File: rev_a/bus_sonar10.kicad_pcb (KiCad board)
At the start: 2 copper layers, 100 x 50 mm, 63 parts, among them J1 POWER_SELECT, J2 TERMINATE_JUMPER, SW1 MJTP1243, U1 LM2940, U2 LTV-826, U3 LTV-826, U4 LTV-826, U5 754410, U6 LM2940, U7 74HCT08, U8 MCP2562, U9 ATMEGA328_DIP28, X1 CRYSTAL

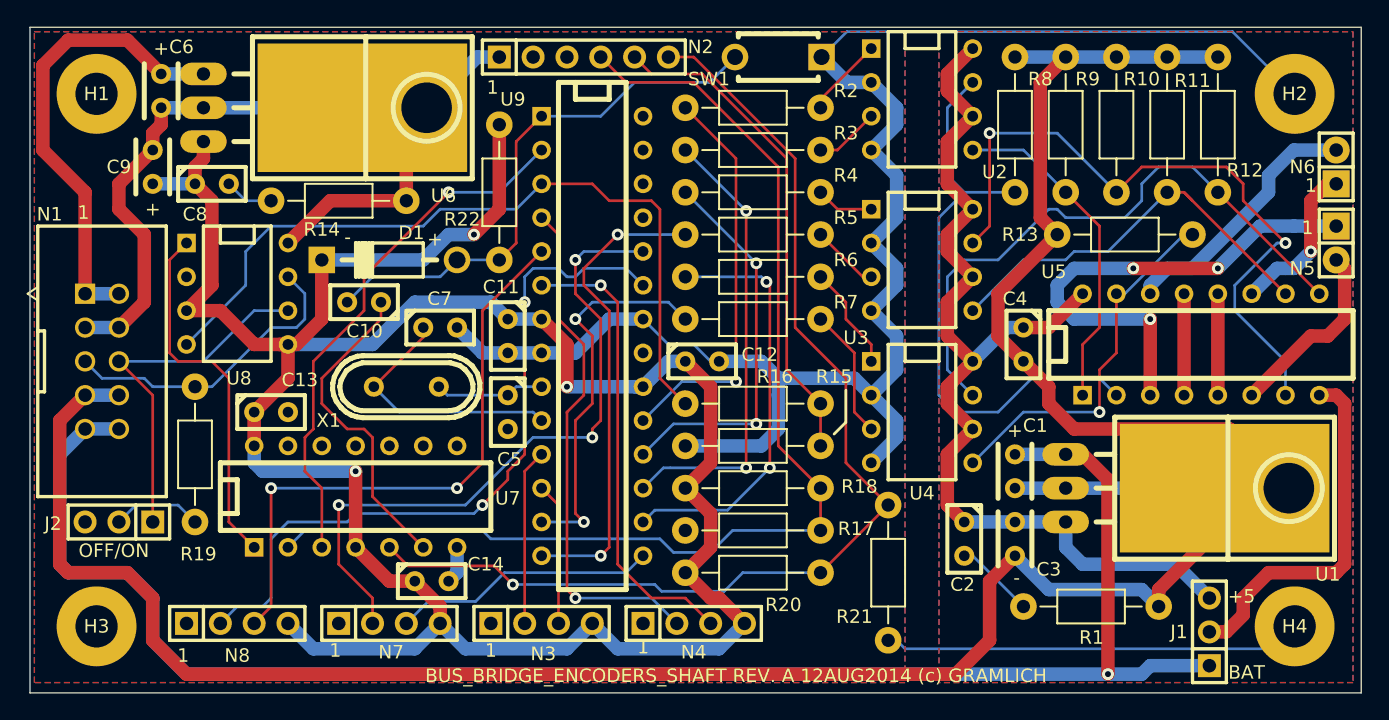
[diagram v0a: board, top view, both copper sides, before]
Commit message: Finnished laying out Rev. A
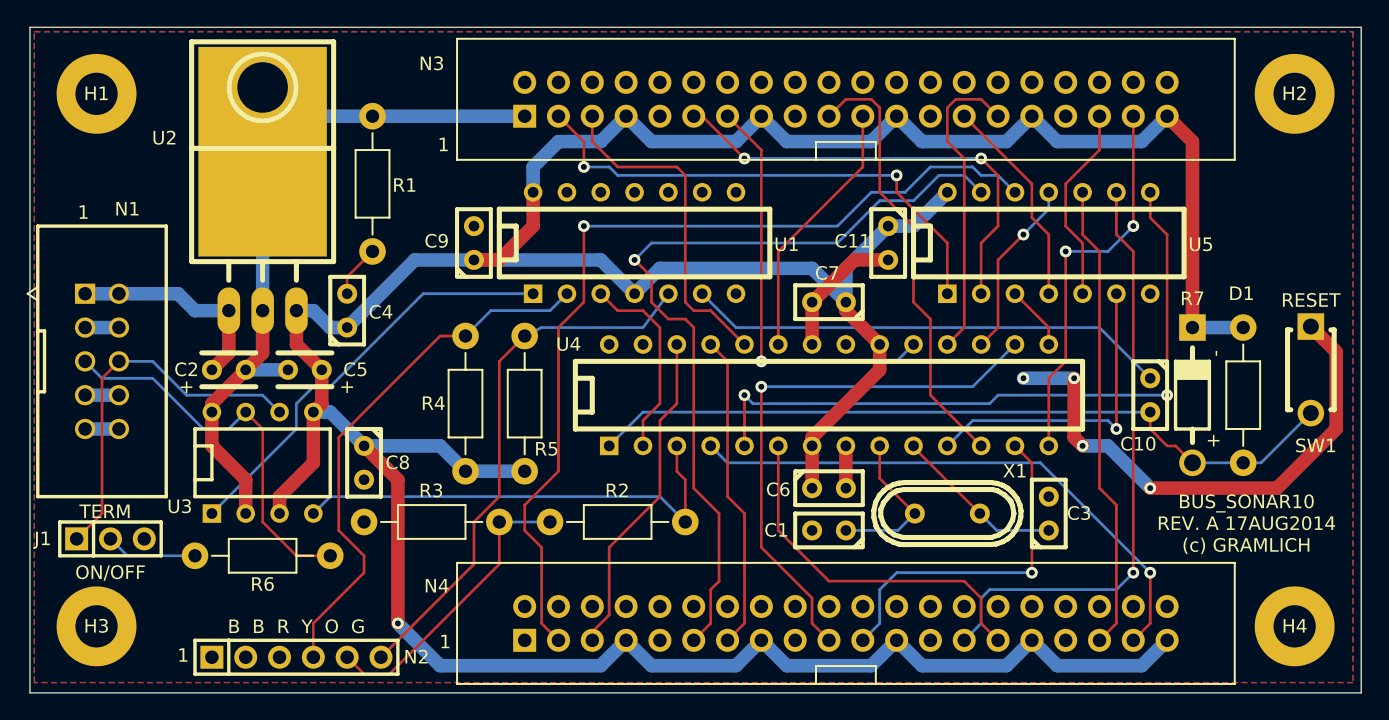
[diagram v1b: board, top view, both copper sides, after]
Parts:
- removed C12, C13, C14: .1uF, Bus_Bridge_Encoders_Sonar_Rev_A:Capacitor3MMDiscRM2.5
- removed J2: TERMINATE_JUMPER, Bus_Bridge_Encoders_Sonar_Rev_A:Pin_Header_Straight_1x03
- removed N5, N6: MOTOR_CONNECTOR, Bus_Bridge_Encoders_Sonar_Rev_A:Pin_Header_Straight_1x02
- removed N7, N8: HC_SR04_CONNECTOR, Bus_Bridge_Encoders_Sonar_Rev_A:Pin_Header_Straight_1x04
- removed R10, R11, R12, R13, R22, R8, R9: 10K, Bus_Bridge_Encoders_Sonar_Rev_A:Resistor_Horizontal_400
- removed R14, R19: .47, Bus_Bridge_Encoders_Sonar_Rev_A:Resistor_Horizontal_400
- removed R15, R17, R20: 22K, Bus_Bridge_Encoders_Sonar_Rev_A:Resistor_Horizontal_400
- removed R16, R18, R21: 33K, Bus_Bridge_Encoders_Sonar_Rev_A:Resistor_Horizontal_400
- removed U6: LM2940, Bus_Bridge_Encoders_Sonar_Rev_A:TO-220_Neutral123_Horizontal_LargePads
- removed U7: 74HCT08, Bus_Bridge_Encoders_Sonar_Rev_A:DIP-14__300
- removed U8: MCP2562, Bus_Bridge_Encoders_Sonar_Rev_A:DIP-8__300
- removed U9: ATMEGA328_DIP28, Bus_Bridge_Encoders_Sonar_Rev_A:DIP-28__300
- C1, C3: value 22uF -> 18pF; footprint Bus_Bridge_Encoders_Sonar_Rev_A:Capacitor4x3RM2-5_RevB -> Bus_Sonar10_Rev_A:Capacitor3MMDiscRM2.5
- C10: value .1uF -> 1uF; footprint Bus_Bridge_Encoders_Sonar_Rev_A:Capacitor3MMDiscRM2.5 -> Bus_Sonar10_Rev_A:Capacitor3MMDiscRM2.5
- C11, C4, C8: footprint Bus_Bridge_Encoders_Sonar_Rev_A:Capacitor3MMDiscRM2.5 -> Bus_Sonar10_Rev_A:Capacitor3MMDiscRM2.5
- C2: value .1uF -> 22uF; footprint Bus_Bridge_Encoders_Sonar_Rev_A:Capacitor3MMDiscRM2.5 -> Bus_Sonar10_Rev_A:Capacitor4x3RM2-5_RevB
- C5: value 18pF -> 22uF; footprint Bus_Bridge_Encoders_Sonar_Rev_A:Capacitor3MMDiscRM2.5 -> Bus_Sonar10_Rev_A:Capacitor4x3RM2-5_RevB
- C6, C9: value 22uF -> .1uF; footprint Bus_Bridge_Encoders_Sonar_Rev_A:Capacitor4x3RM2-5_RevB -> Bus_Sonar10_Rev_A:Capacitor3MMDiscRM2.5
- C7: value 18pF -> .1uF; footprint Bus_Bridge_Encoders_Sonar_Rev_A:Capacitor3MMDiscRM2.5 -> Bus_Sonar10_Rev_A:Capacitor3MMDiscRM2.5
- D1: footprint Bus_Bridge_Encoders_Sonar_Rev_A:Diode_DO-41_SOD81_Horizontal_RM10 -> Bus_Sonar10_Rev_A:Diode_DO-41_SOD81_Horizontal_RM10
- G1: footprint Bus_Bridge_Encoders_Sonar_Rev_A:OSHW_LOGO_400mil -> Bus_Sonar10_Rev_A:OSHW_LOGO_400mil
- H1, H2, H3, H4: footprint Bus_Bridge_Encoders_Sonar_Rev_A:MountingHole_3mm -> Bus_Sonar10_Rev_A:MountingHole_3mm
- J1: value POWER_SELECT -> TERMINATE_JUMPER; footprint Bus_Bridge_Encoders_Sonar_Rev_A:Pin_Header_Straight_1x03 -> Bus_Sonar10_Rev_A:Pin_Header_Straight_1x03
- N1: footprint Bus_Bridge_Encoders_Sonar_Rev_A:Pin_Header_Straight_2x05_Shrouded -> Bus_Sonar10_Rev_A:Pin_Header_Straight_2x05_Shrouded
- N2: footprint Bus_Bridge_Encoders_Sonar_Rev_A:Pin_Header_Straight_1x06 -> Bus_Sonar10_Rev_A:Pin_Header_Straight_1x06
- N3, N4: value ENCODER_CONNECTOR -> 302-S401; footprint Bus_Bridge_Encoders_Sonar_Rev_A:Pin_Header_Straight_1x04 -> Bus_Sonar10_Rev_A:Pin_Header_Straight_2x20_Shrouded
- R1: footprint Bus_Bridge_Encoders_Sonar_Rev_A:Resistor_Horizontal_400 -> Bus_Sonar10_Rev_A:Resistor_Horizontal_400
- R2: value 470 -> 22K; footprint Bus_Bridge_Encoders_Sonar_Rev_A:Resistor_Horizontal_400 -> Bus_Sonar10_Rev_A:Resistor_Horizontal_400
- R3: value 470 -> 33K; footprint Bus_Bridge_Encoders_Sonar_Rev_A:Resistor_Horizontal_400 -> Bus_Sonar10_Rev_A:Resistor_Horizontal_400
- R4, R5: value 470 -> 100K; footprint Bus_Bridge_Encoders_Sonar_Rev_A:Resistor_Horizontal_400 -> Bus_Sonar10_Rev_A:Resistor_Horizontal_400
- R6: value 470 -> .47; footprint Bus_Bridge_Encoders_Sonar_Rev_A:Resistor_Horizontal_400 -> Bus_Sonar10_Rev_A:Resistor_Horizontal_400
- R7: value 470 -> 10K; footprint Bus_Bridge_Encoders_Sonar_Rev_A:Resistor_Horizontal_400 -> Bus_Sonar10_Rev_A:Resistor_Horizontal_400
- SW1: footprint Bus_Bridge_Encoders_Sonar_Rev_A:Button_6.5MM -> Bus_Sonar10_Rev_A:Button_6.5MM
- U1: value LM2940 -> 74HCT08; footprint Bus_Bridge_Encoders_Sonar_Rev_A:TO-220_Neutral123_Horizontal_LargePads -> Bus_Sonar10_Rev_A:DIP-14__300
- U2: value LTV-826 -> LM2940; footprint Bus_Bridge_Encoders_Sonar_Rev_A:DIP-8__300 -> Bus_Sonar10_Rev_A:TO-220_Neutral123_Horizontal_LargePads
- U3: value LTV-826 -> MCP2562; footprint Bus_Bridge_Encoders_Sonar_Rev_A:DIP-8__300 -> Bus_Sonar10_Rev_A:DIP-8__300
- U4: value LTV-826 -> ATMEGA328_DIP28; footprint Bus_Bridge_Encoders_Sonar_Rev_A:DIP-8__300 -> Bus_Sonar10_Rev_A:DIP-28__300
- U5: value 754410 -> 74HCT32; footprint Bus_Bridge_Encoders_Sonar_Rev_A:DIP-16__300 -> Bus_Sonar10_Rev_A:DIP-14__300
- X1: footprint Bus_Bridge_Encoders_Sonar_Rev_A:Crystal_HC49-U_Vertical -> Bus_Sonar10_Rev_A:Crystal_HC49-U_Vertical
- moved J1 82.8 mm to (106.0, 138.4), turned to 0 degrees
- moved R1 62.6 mm to (125.7, 111.8), turned to 270 degrees
- moved D1 61.2 mm to (187.3, 127.6), turned to 90 degrees
- moved C10 59.5 mm to (184.2, 127.6), turned to 270 degrees
- moved C6 58.4 mm to (160.0, 134.6), turned to 0 degrees
- moved C2 56.7 mm to (114.9, 125.7), turned to 0 degrees
- moved U2 52.0 mm to (117.5, 121.3), turned to 0 degrees
- moved U3 51.8 mm to (117.5, 132.7), turned to 0 degrees
- moved C4 50.9 mm to (123.8, 121.3), turned to 90 degrees
- moved N2 50.0 mm to (120.0, 147.3)
- moved SW1 46.4 mm to (196.2, 125.7), turned to 270 degrees
- moved N3 45.5 mm to (161.3, 105.4)
- moved R6 42.4 mm to (117.5, 139.7), turned to 180 degrees
- moved X1 41.7 mm to (168.9, 136.5), turned to 0 degrees
- moved R7 37.3 mm to (191.1, 127.6), turned to 90 degrees
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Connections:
- C1 pad 1: /BPWR -> Net-(C1-Pad1)
- C1 pad 2: /BGND -> GND
- C2 pad 1: /M5V -> /LPWR
- C2 pad 2: Net-(C2-Pad2) -> GND
- C3 pad 1: /M5V -> Net-(C3-Pad1)
- C3 pad 2: /BGND -> GND
- C4 pad 1: /M5V -> +5V
- C4 pad 2: /BGND -> Net-(C4-Pad2)
- C5 pad 1: Net-(C5-Pad1) -> +5V
- C6 pad 1: /LPWR -> +5V
- C7 pad 1: Net-(C7-Pad1) -> +5V
- C8 pad 2: Net-(C8-Pad2) -> GND
- J1 pad 1: /BPWR -> Net-(J1-Pad1)
- J1 pad 2: /MOTOR_POWER -> Net-(J1-Pad2)
- J1 pad 3: /M5V -> Net-(J1-Pad3)
- N1 pad 10: /BPWR -> Net-(N1-Pad10)
- N1 pad 6: Net-(J2-Pad1) -> Net-(J1-Pad1)
- N1 pad 7: /BGND -> Net-(N1-Pad7)
- N1 pad 8: /BGND -> Net-(N1-Pad7)
- N1 pad 9: /BPWR -> Net-(N1-Pad10)
- N3 pad 2: /D5 -> GND
- N3 pad 3: /D6 -> Net-(N3-Pad3)
- N3 pad 4: +5V -> GND
- N4 pad 2: /D2 -> GND
- N4 pad 3: /D4 -> Net-(N4-Pad3)
- N4 pad 4: +5V -> GND
- R1 pad 1: /BGND -> GND
- R1 pad 2: Net-(C2-Pad2) -> Net-(C4-Pad2)
- R2 pad 1: /D13 -> Net-(N2-Pad5)
- R2 pad 2: Net-(R2-Pad2) -> /TXD
- R3 pad 1: /D11 -> GND
- R3 pad 2: Net-(R3-Pad2) -> Net-(N2-Pad5)
- R4 pad 1: /D12 -> Net-(N2-Pad4)
- R4 pad 2: Net-(R4-Pad2) -> +5V
- R5 pad 1: /D8 -> Net-(N2-Pad6)
- R5 pad 2: Net-(R5-Pad2) -> +5V
- R6 pad 1: /D10 -> Net-(N1-Pad5)
- R6 pad 2: Net-(R6-Pad2) -> Net-(J1-Pad2)
- R7 pad 1: /D7 -> /~RESET
- R7 pad 2: Net-(R7-Pad2) -> +5V
- U1 pad 1: /BPWR -> Net-(U1-Pad1)
- U1 pad 2: /BGND -> Net-(N2-Pad4)
- U1 pad 3: /M5V -> /RXD
- U2 pad 1: Net-(R2-Pad2) -> /LPWR
- U2 pad 3: Net-(R3-Pad2) -> +5V
- U3 pad 1: Net-(R4-Pad2) -> Net-(U1-Pad1)
- U3 pad 3: Net-(R5-Pad2) -> +5V
- U3 pad 4: GND -> /TXD
- U3 pad 5: Net-(R11-Pad2) -> +5V
- U3 pad 6: /M5V -> Net-(J1-Pad1)
- U3 pad 7: Net-(R10-Pad2) -> Net-(N1-Pad5)
- U3 pad 8: /M5V -> GND
- U4 pad 1: Net-(R6-Pad2) -> /~RESET
- U4 pad 2: GND -> /RXD
- U4 pad 3: Net-(R7-Pad2) -> /TXD
- U4 pad 4: GND -> /D2
- U4 pad 5: Net-(R13-Pad2) -> /D3
- U4 pad 6: /M5V -> /D4
- U4 pad 7: Net-(R12-Pad2) -> +5V
- U4 pad 8: /M5V -> GND
- U5 pad 1: Net-(R9-Pad2) -> Net-(N3-Pad3)
- U5 pad 10: Net-(R11-Pad2) -> Net-(N4-Pad35)
- U5 pad 11: /M2+ -> /D11
- U5 pad 12: /BGND -> Net-(N4-Pad3)
- U5 pad 13: /BGND -> Net-(N4-Pad11)
- U5 pad 14: /M2- -> +5V
- U5 pad 2: Net-(R8-Pad2) -> Net-(N3-Pad11)
- U5 pad 3: /M1+ -> /D9
- U5 pad 4: /BGND -> Net-(N3-Pad27)
- U5 pad 5: /BGND -> Net-(N3-Pad35)
- U5 pad 6: /M1- -> /D5
- U5 pad 7: Net-(R10-Pad2) -> GND
- U5 pad 8: /MOTOR_POWER -> /D3
- U5 pad 9: Net-(R12-Pad2) -> Net-(N4-Pad27)
- X1 pad 1: Net-(C5-Pad1) -> Net-(C1-Pad1)
- X1 pad 2: Net-(C7-Pad1) -> Net-(C3-Pad1)
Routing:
- net /BGND: track 228.4 -> 0.00 mm
- net /BPWR: track 127.8 -> 0.00 mm, vias 1 -> 0
- net GND: track 226.9 -> 116.5 mm, vias 0 -> 4
- net +5V: track 190.0 -> 278.7 mm, vias 3 -> 1
- net /M5V: track 77.0 -> 0.00 mm
- net Net-(N4-Pad3): track 0.00 -> 69.0 mm, vias 0 -> 1
- net Net-(N4-Pad11): track 0.00 -> 61.9 mm, vias 0 -> 1
- net /A0: track 54.6 -> 0.00 mm, vias 2 -> 0
- net Net-(R10-Pad2): track 51.7 -> 0.00 mm, vias 2 -> 0
- net /A1: track 50.8 -> 0.00 mm, vias 3 -> 0
- net Net-(N2-Pad4): track 87.3 -> 40.5 mm
- net Net-(R12-Pad2): track 46.3 -> 0.00 mm
- net Net-(N4-Pad27): track 0.00 -> 45.0 mm, vias 0 -> 1
- net Net-(R8-Pad2): track 44.8 -> 0.00 mm
- net Net-(N2-Pad6): track 83.1 -> 40.8 mm, vias 1 -> 0
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- removed copper zone on B.Cu, net /BGND
- removed copper zone on F.Cu, net /BGND
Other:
- board text added: "B B R Y O G"
- board text added: "BUS_SONAR10 REV. A 17AUG2014 (c) GRAMLICH"
- board text added: "ON/OFF"
- board text added: "RESET"
- board text added: "TERM"
- board text removed: "+5"
- board text removed: "-"
- board text removed: "BAT"
- board text removed: "BUS_BRIDGE_ENCODERS_SHAFT REV. A 12AUG2014 (c) GRAMLICH"
- board text removed: "OFF/ON"
